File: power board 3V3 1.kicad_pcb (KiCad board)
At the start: 2 copper layers, 66 x 90 mm, 29 parts, among them J1 UVLO TP, J2 CHRGR TP, J3 BATT & RPP TP, J4 LDO TP, J5 SRC CTRL TP, Q1 NMOS - HL3400A, Q2 PMOS - SI2301, Q3 PMOS - SI2301, U1 TP4056-42-ESOP8, U2 HT7533-1-SOT89, U3 LM358DR

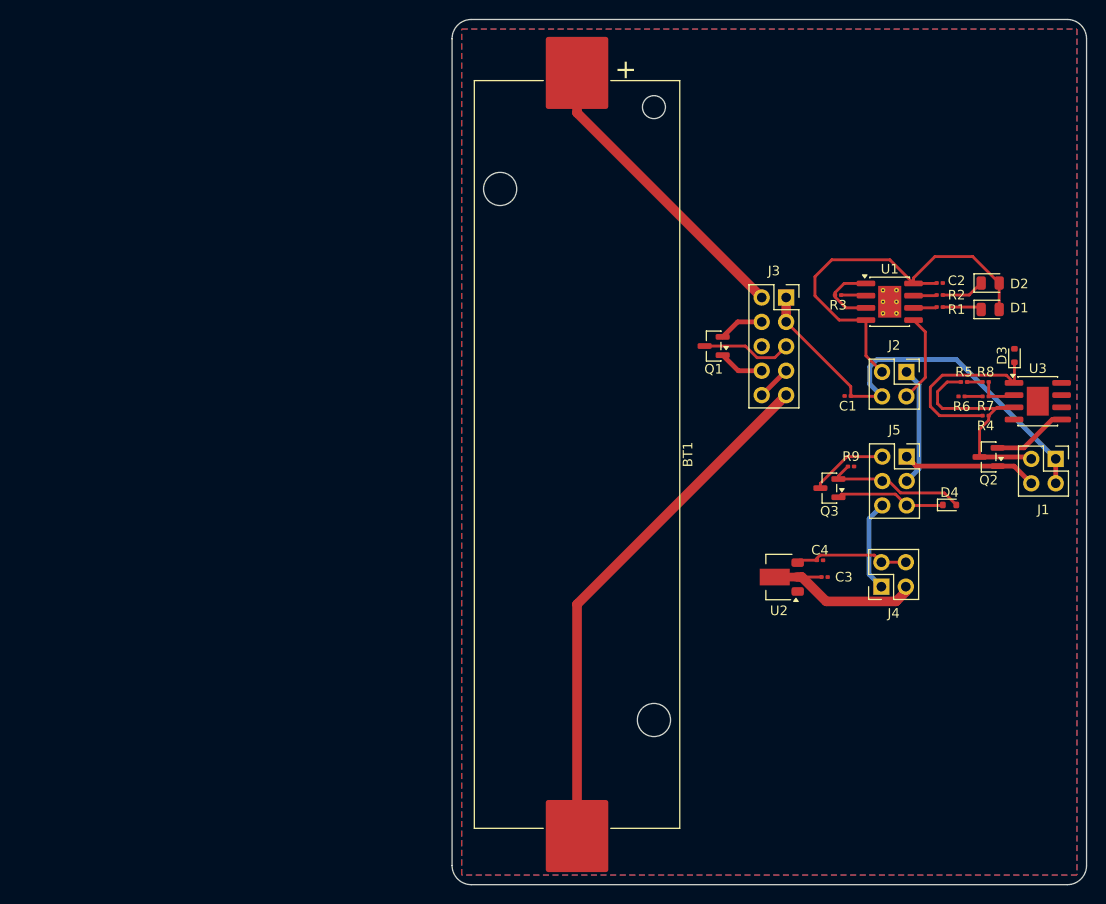
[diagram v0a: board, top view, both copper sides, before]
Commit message: PCB looks better now
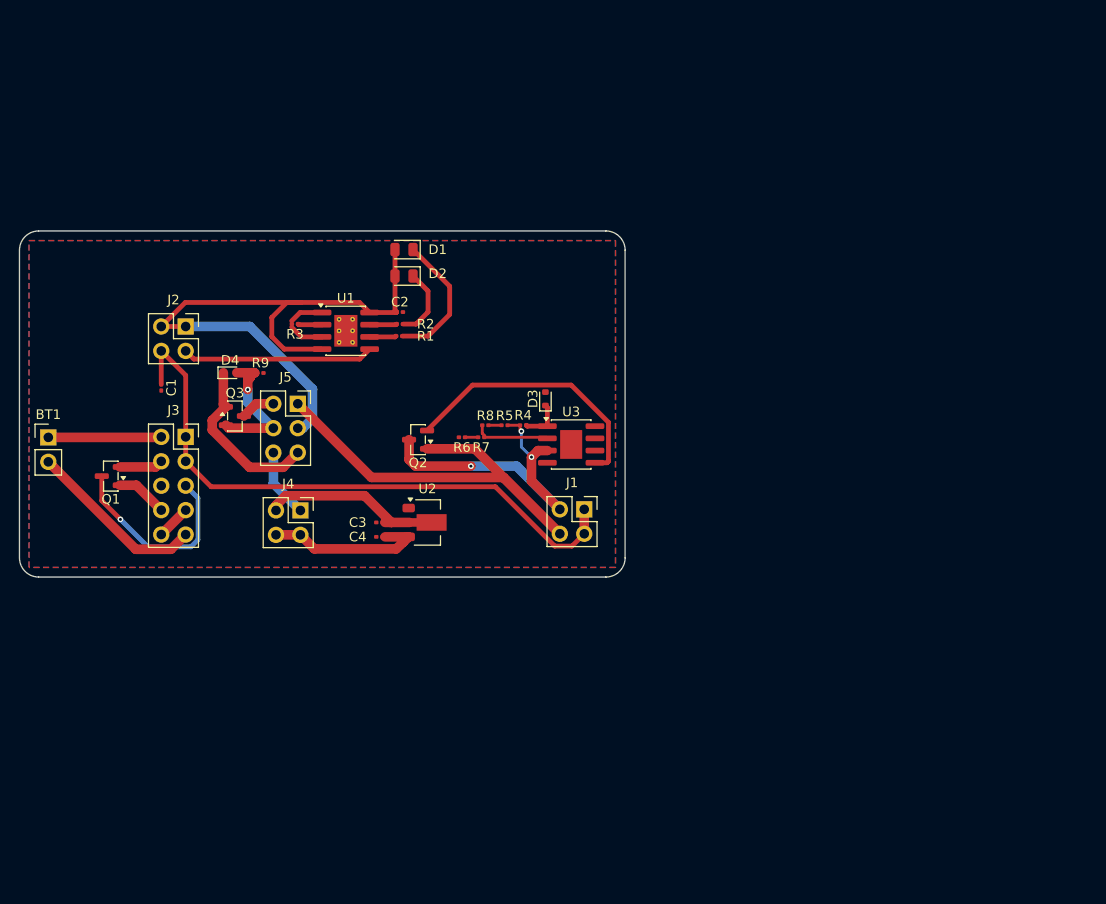
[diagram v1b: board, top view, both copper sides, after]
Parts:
- BT1: footprint Battery:BatteryHolder_Keystone_1042_1x18650 -> Connector_PinHeader_2.54mm:PinHeader_1x02_P2.54mm_Vertical
- moved D4 76.1 mm to (60.9, 66.8)
- moved J2 75.1 mm to (56.3, 61.9)
- moved C1 71.4 mm to (53.8, 68.3), turned to -90 degrees
- moved Q1 64.2 mm to (48.5, 77.5)
- moved J3 64.1 mm to (56.3, 73.4)
- moved J5 63.6 mm to (68.0, 70.0)
- moved Q3 62.3 mm to (61.4, 71.2), turned to 0 degrees
- moved R9 62.2 mm to (64.1, 66.8)
- moved D1 61.3 mm to (79.0, 53.9), turned to 180 degrees
- moved D2 61.0 mm to (79.0, 56.7), turned to 180 degrees
- moved J4 61.0 mm to (68.2, 81.1), turned to 0 degrees
- moved Q2 59.4 mm to (80.5, 73.7)
- moved U1 56.7 mm to (73.0, 62.4)
- moved R3 56.6 mm to (67.7, 61.7)
- moved R1 56.3 mm to (78.5, 62.9)
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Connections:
- C2 pad 1: /POW CHRGR2 -> +5V
- D1 pad 2: /POW CHRGR2 -> +5V
- D2 pad 2: /POW CHRGR2 -> +5V
- J2 pad 2: /POW CHRGR2 -> +5V
- U1 pad 4: /POW CHRGR2 -> +5V
- U1 pad 8: /POW CHRGR2 -> +5V
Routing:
- net +5V: track 12.4 -> 67.4 mm
- net /POW CHRGR2: track 43.1 -> 0.00 mm
- net /+BATT_UVLO: track 14.1 -> 50.3 mm
- net /-BATT1: track 54.9 -> 18.7 mm
- net Net-(Q2-G): track 7.87 -> 28.0 mm
- net /+BATT2: track 31.3 -> 11.8 mm
- net +BATT: track 46.4 -> 64.2 mm
- net /Vref: track 19.5 -> 4.45 mm
- net /RPPGND1: track 9.47 -> 21.0 mm, vias 0 -> 1
- net /BATT2CHRG1: track 9.25 -> 19.9 mm
- net Net-(D1-K): track 4.10 -> 14.2 mm
- net /UVLO ON2: track 25.4 -> 33.6 mm, vias 0 -> 3
- net /SELECTOR OUT1: track 11.5 -> 17.8 mm
- net +3V3: track 12.0 -> 17.4 mm
- net /UVLO2SEL2: track 8.09 -> 3.59 mm
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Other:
- board size 66 x 90 mm -> 63 x 36 mm
